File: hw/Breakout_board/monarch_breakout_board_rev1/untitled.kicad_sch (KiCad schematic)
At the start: 10 parts, among them J1 5037630491, J2 5037630291, J3 5037630291, J4 5037630291, J5 5037630291, J6 5037630291

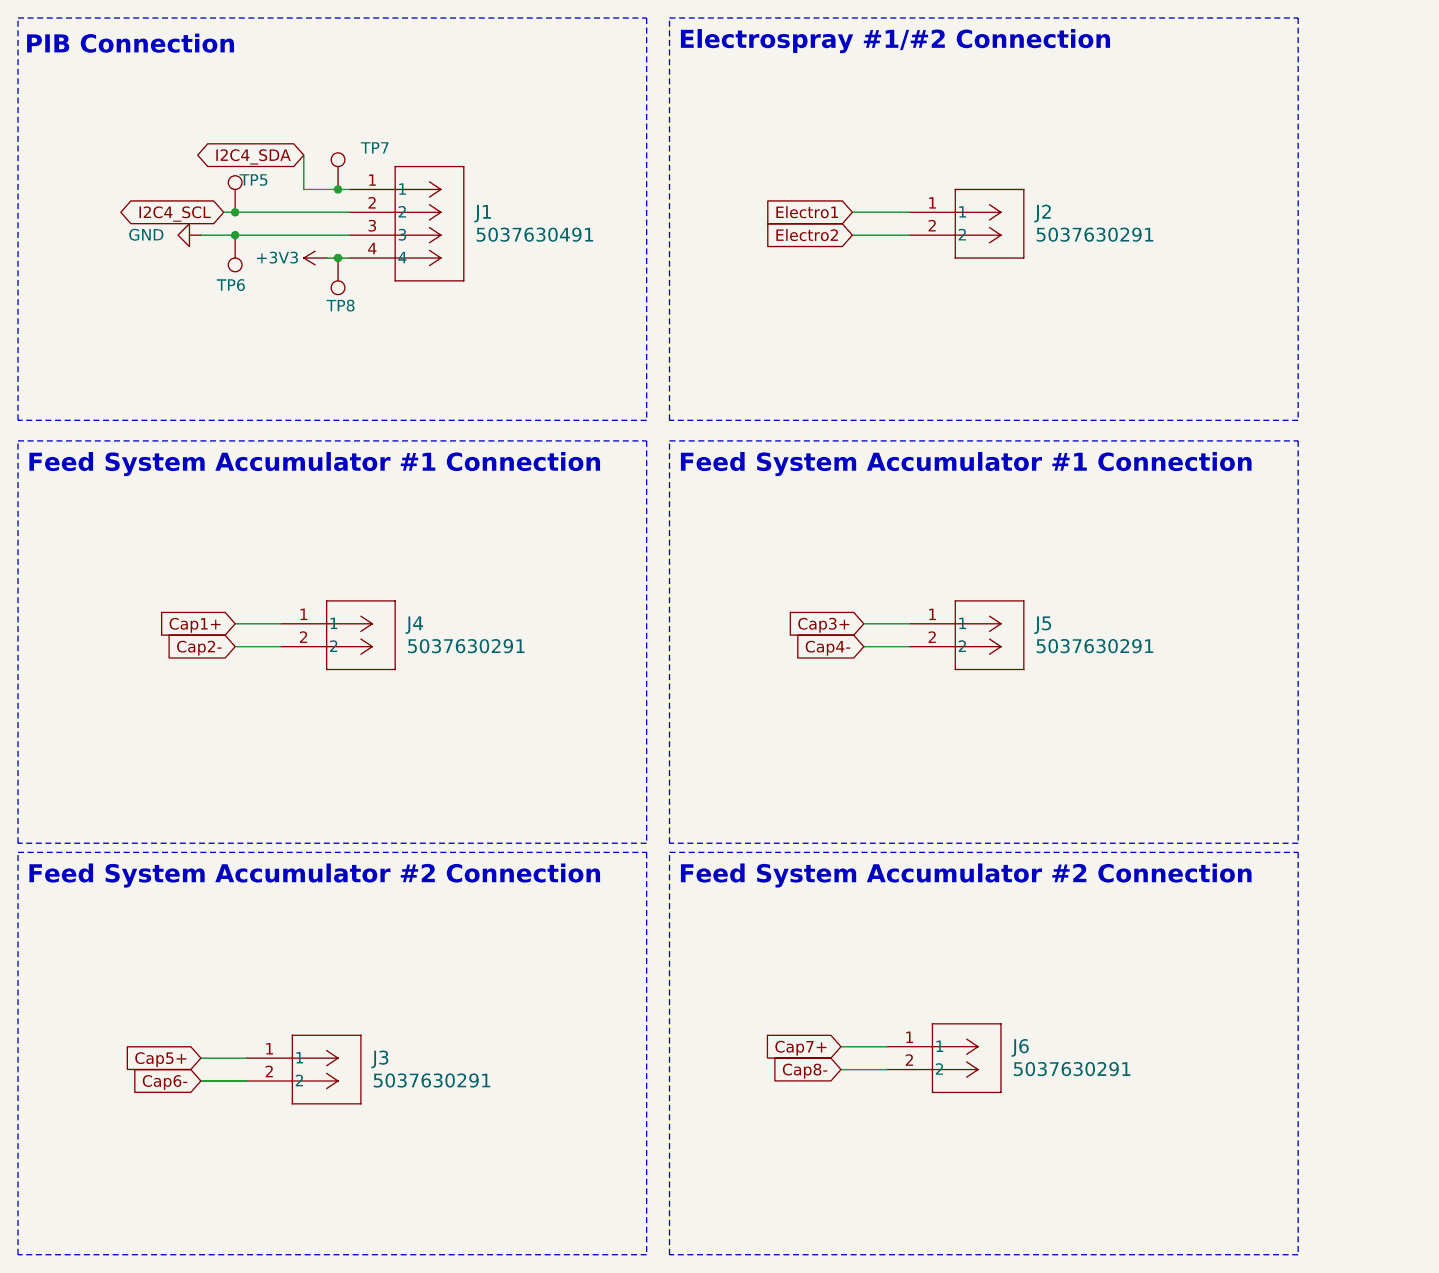
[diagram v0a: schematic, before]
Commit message: Revert "Crystal Clock Completion, All Pins Assigned, More Routing Work"
This reverts commit 432819c756e1f3cf9abb2627b488983cb7a3cfe3
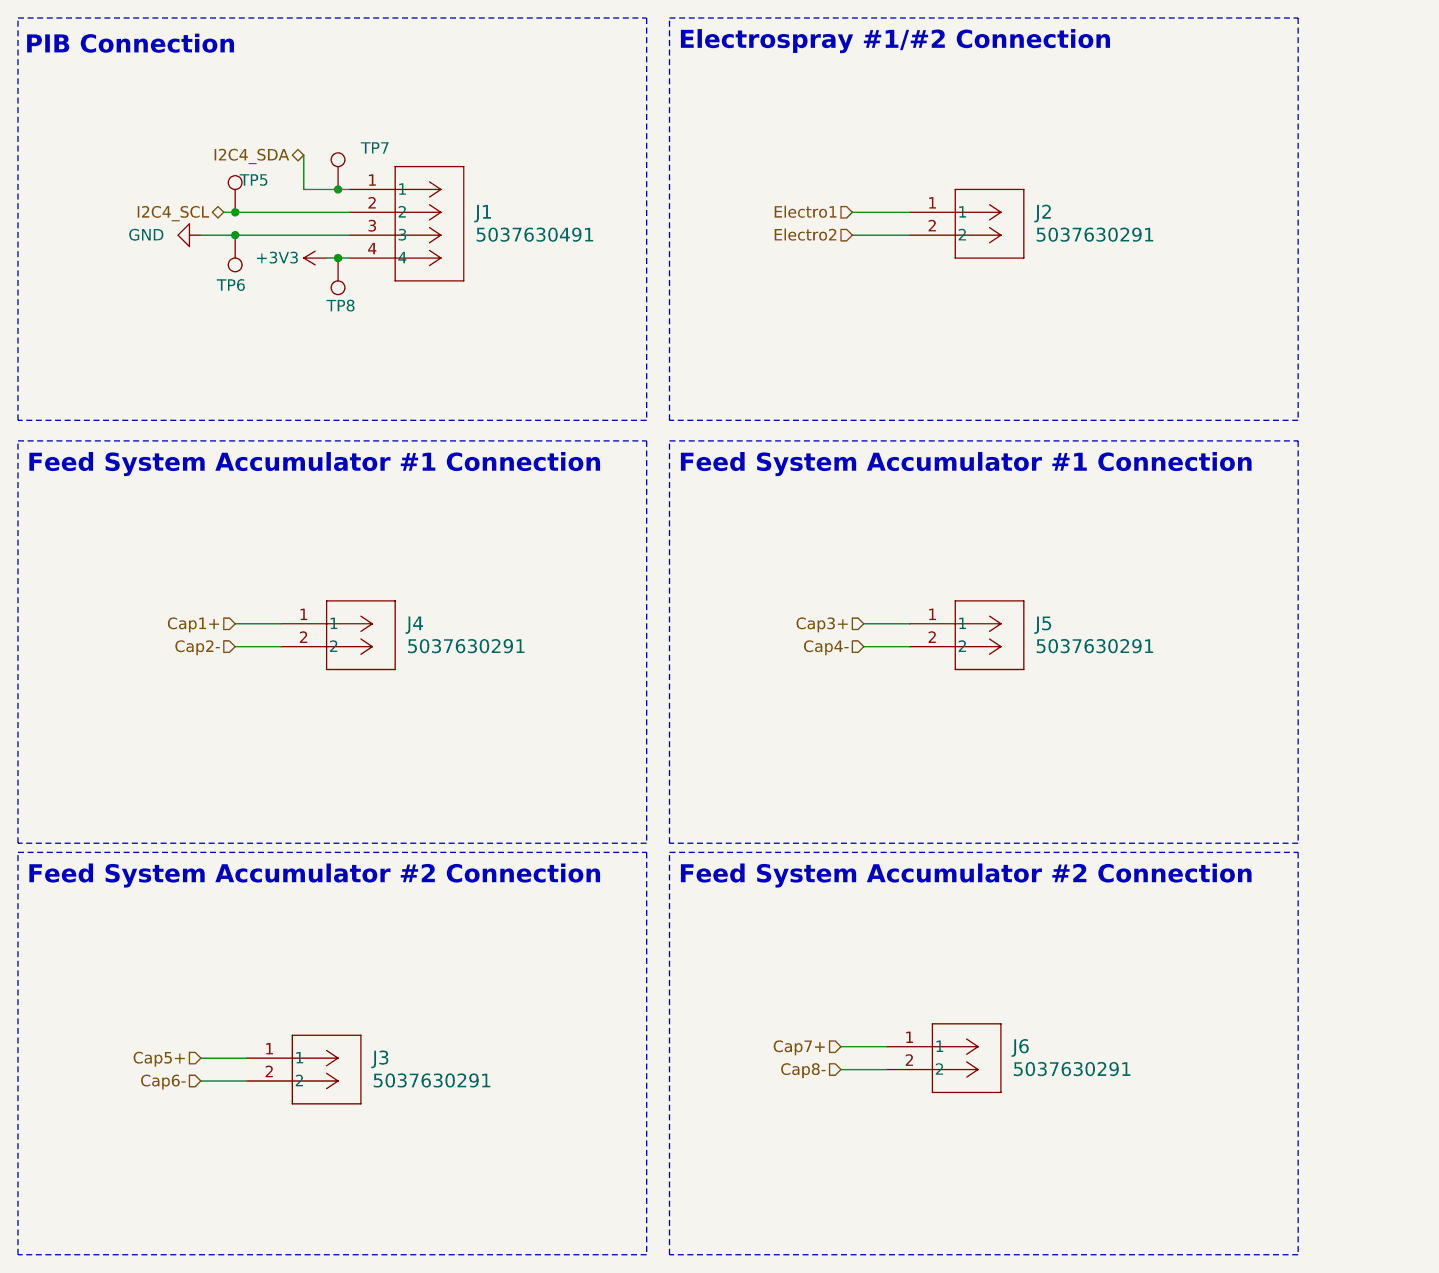
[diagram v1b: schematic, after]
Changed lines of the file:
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@@
 		)
 	)
-	(global_label "Cap1+"
+	(hierarchical_label "Cap5+"
 		(shape input)
-		(at 39.37 81.28 180)
-		(fields_autoplaced yes)
+		(at 35.56 129.54 180)
 		(effects
 			(font
@@
 			(justify right)
 		)
-		(property "Intersheetrefs" "${INTERSHEET_REFS}"
-			(at 30.0349 81.28 0)
-			(effects
-				(font
-					(size 1.27 1.27)
-				)
-				(justify right)
-				(hide yes)
-			)
-		)
 	)
-	(global_label "Electro2"
+	(hierarchical_label "Cap4-"
 		(shape input)
-		(at 107.95 38.1 180)
-		(fields_autoplaced yes)
+		(at 109.22 83.82 180)
 		(effects
 			(font
@@
 			(justify right)
 		)
-		(property "Intersheetrefs" "${INTERSHEET_REFS}"
-			(at 97.103 38.1 0)
-			(effects
-				(font
-					(size 1.27 1.27)
-				)
-				(justify right)
-				(hide yes)
-			)
-		)
 	)
-	(global_label "Cap4-"
-		(shape input)
-		(at 109.22 83.82 180)
-		(fields_autoplaced yes)
+	(hierarchical_label "I2C4_SCL"
+		(shape bidirectional)
+		(at 38.1 35.56 180)
 		(effects
 			(font
@@
 			(justify right)
 		)
-		(property "Intersheetrefs" "${INTERSHEET_REFS}"
-			(at 99.8849 83.82 0)
-			(effects
-				(font
-					(size 1.27 1.27)
-				)
-				(justify right)
-				(hide yes)
-			)
-		)
 	)
-	(global_label "Cap7+"
+	(hierarchical_label "Cap3+"
 		(shape input)
-		(at 106.68 128.27 180)
-		(fields_autoplaced yes)
+		(at 109.22 81.28 180)
 		(effects
 			(font
@@
 			(justify right)
 		)
-		(property "Intersheetrefs" "${INTERSHEET_REFS}"
-			(at 97.3449 128.27 0)
-			(effects
-				(font
-					(size 1.27 1.27)
-				)
-				(justify right)
-				(hide yes)
-			)
-		)
 	)
-	(global_label "Electro1"
+	(hierarchical_label "Electro2"
 		(shape input)
-		(at 107.95 35.56 180)
-		(fields_autoplaced yes)
+		(at 107.95 38.1 180)
 		(effects
 			(font
@@
 			(justify right)
 		)
-		(property "Intersheetrefs" "${INTERSHEET_REFS}"
-			(at 97.103 35.56 0)
-			(effects
-				(font
-					(size 1.27 1.27)
-				)
-				(justify right)
-				(hide yes)
-			)
-		)
 	)
-	(global_label "I2C4_SDA"
-		(shape bidirectional)
-		(at 46.99 29.21 180)
-		(fields_autoplaced yes)
+	(hierarchical_label "Cap2-"
+		(shape input)
+		(at 39.37 83.82 180)
 		(effects
 			(font
@@
 			(justify right)
 		)
-		(property "Intersheetrefs" "${INTERSHEET_REFS}"
-			(at 34.064 29.21 0)
-			(effects
-				(font
-					(size 1.27 1.27)
-				)
-				(justify right)
-				(hide yes)
-			)
-		)
 	)
-	(global_label "Cap3+"
+	(hierarchical_label "Cap6-"
 		(shape input)
-		(at 109.22 81.28 180)
-		(fields_autoplaced yes)
+		(at 35.56 132.08 180)
 		(effects
 			(font
@@
 			(justify right)
 		)
-		(property "Intersheetrefs" "${INTERSHEET_REFS}"
-			(at 99.8849 81.28 0)
-			(effects
-				(font
-					(size 1.27 1.27)
-				)
-				(justify right)
-				(hide yes)
-			)
-		)
 	)
-	(global_label "I2C4_SCL"
-		(shape bidirectional)
-		(at 38.1 35.56 180)
-		(fields_autoplaced yes)
+	(hierarchical_label "Cap8-"
+		(shape input)
+		(at 106.68 130.81 180)
 		(effects
 			(font
@@
 			(justify right)
 		)
-		(property "Intersheetrefs" "${INTERSHEET_REFS}"
-			(at 25.2345 35.56 0)
-			(effects
-				(font
-					(size 1.27 1.27)
-				)
-				(justify right)
-				(hide yes)
-			)
-		)
 	)
-	(global_label "Cap2-"
+	(hierarchical_label "Electro1"
 		(shape input)
-		(at 39.37 83.82 180)
-		(fields_autoplaced yes)
+		(at 107.95 35.56 180)
 		(effects
 			(font
@@
 			(justify right)
 		)
-		(property "Intersheetrefs" "${INTERSHEET_REFS}"
-			(at 30.0349 83.82 0)
-			(effects
-				(font
-					(size 1.27 1.27)
-				)
-				(justify right)
-				(hide yes)
-			)
-		)
 	)
-	(global_label "Cap5+"
+	(hierarchical_label "Cap7+"
 		(shape input)
-		(at 35.56 129.54 180)
-		(fields_autoplaced yes)
+		(at 106.68 128.27 180)
 		(effects
 			(font
@@
 			(justify right)
 		)
-		(property "Intersheetrefs" "${INTERSHEET_REFS}"
-			(at 26.2249 129.54 0)
-			(effects
-				(font
-					(size 1.27 1.27)
-				)
-				(justify right)
-				(hide yes)
-			)
-		)
 	)
-	(global_label "Cap8-"
+	(hierarchical_label "Cap1+"
 		(shape input)
-		(at 106.68 130.81 180)
-		(fields_autoplaced yes)
+		(at 39.37 81.28 180)
 		(effects
 			(font
@@
 			(justify right)
 		)
-		(property "Intersheetrefs" "${INTERSHEET_REFS}"
-			(at 97.3449 130.81 0)
-			(effects
-				(font
-					(size 1.27 1.27)
-				)
-				(justify right)
-				(hide yes)
-			)
-		)
 	)
-	(global_label "Cap6-"
-		(shape input)
-		(at 35.56 132.08 180)
-		(fields_autoplaced yes)
+	(hierarchical_label "I2C4_SDA"
+		(shape bidirectional)
+		(at 46.99 29.21 180)
 		(effects
 			(font
@@
 			(justify right)
 		)
-		(property "Intersheetrefs" "${INTERSHEET_REFS}"
-			(at 26.2249 132.08 0)
-			(effects
-				(font
-					(size 1.27 1.27)
-				)
-				(justify right)
-				(hide yes)
-			)
-		)
 	)

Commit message: Breakout Board History Fix
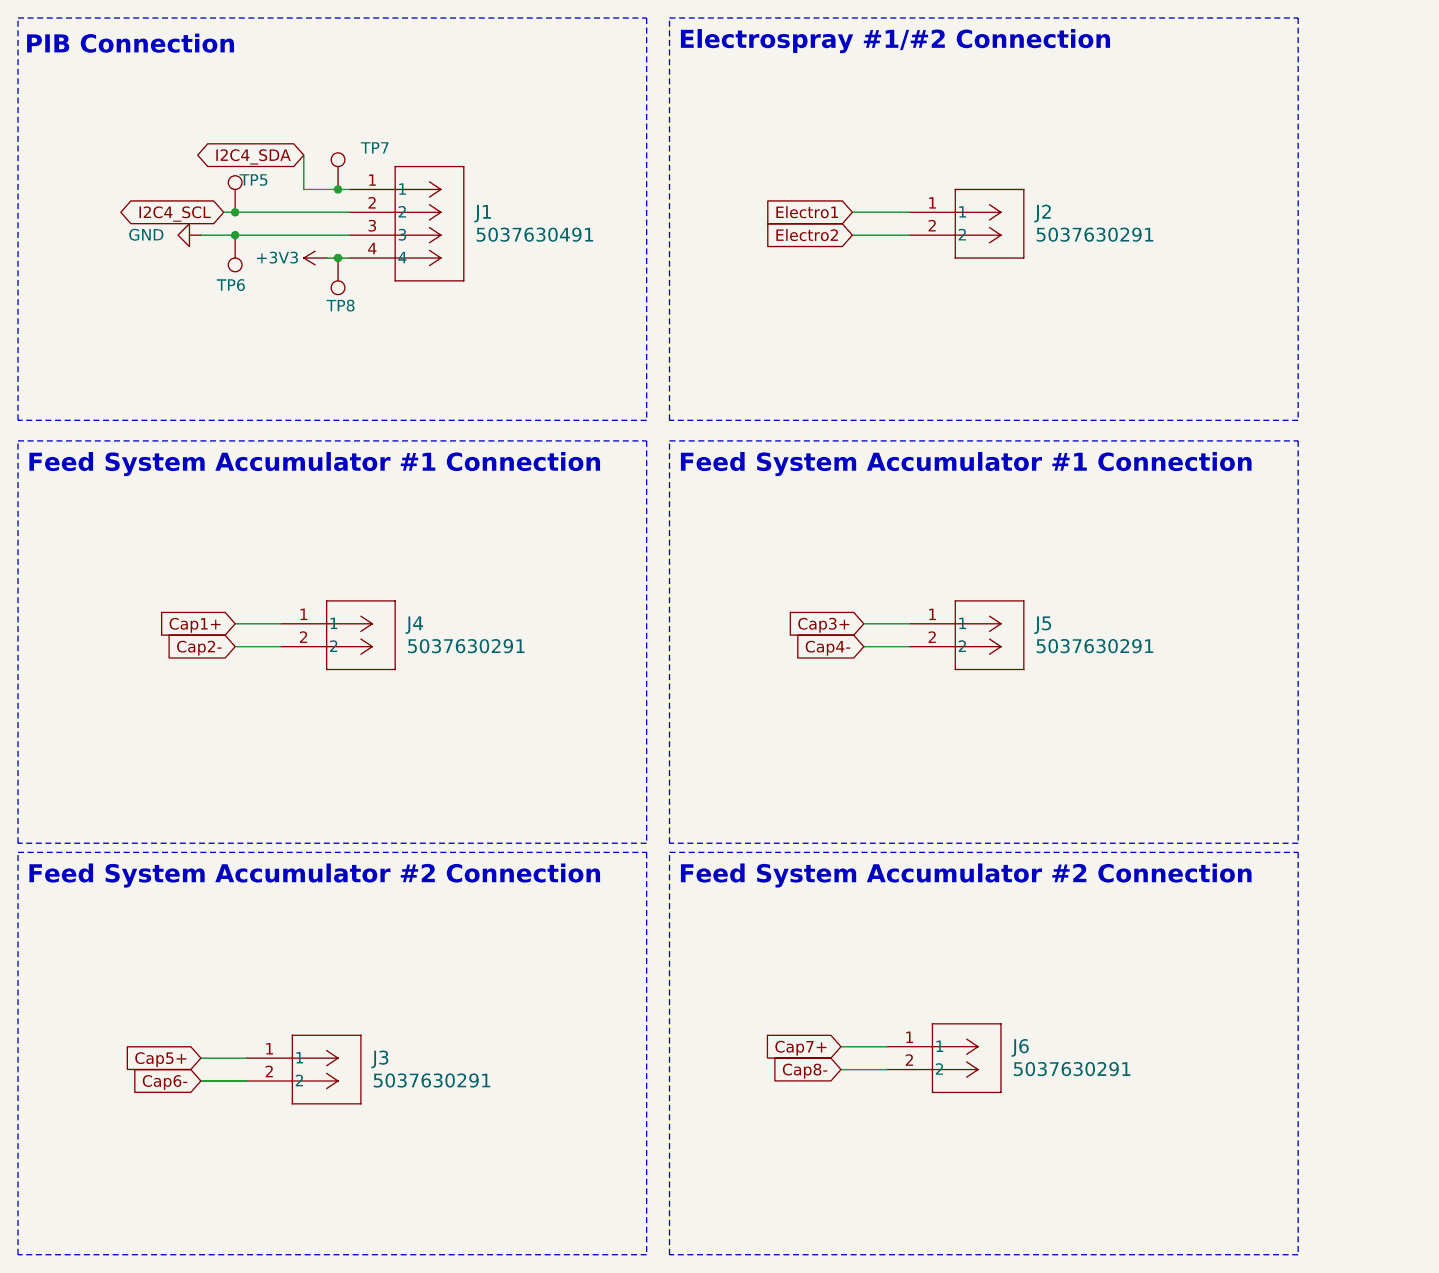
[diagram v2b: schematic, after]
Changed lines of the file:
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@@
 		)
 	)
-	(hierarchical_label "Cap5+"
-		(shape input)
-		(at 35.56 129.54 180)
-		(effects
-			(font
-				(size 1.27 1.27)
-			)
-			(justify right)
-		)
-	)
-	(hierarchical_label "Cap4-"
+	(global_label "Cap1+"
+		(shape input)
+		(at 39.37 81.28 180)
+		(fields_autoplaced yes)
+		(effects
+			(font
+				(size 1.27 1.27)
+			)
+			(justify right)
+		)
+		(property "Intersheetrefs" "${INTERSHEET_REFS}"
+			(at 30.0349 81.28 0)
+			(effects
+				(font
+					(size 1.27 1.27)
+				)
+				(justify right)
+				(hide yes)
+			)
+		)
+	)
+	(global_label "Electro2"
+		(shape input)
+		(at 107.95 38.1 180)
+		(fields_autoplaced yes)
+		(effects
+			(font
+				(size 1.27 1.27)
+			)
+			(justify right)
+		)
+		(property "Intersheetrefs" "${INTERSHEET_REFS}"
+			(at 97.103 38.1 0)
+			(effects
+				(font
+					(size 1.27 1.27)
+				)
+				(justify right)
+				(hide yes)
+			)
+		)
+	)
+	(global_label "Cap4-"
 		(shape input)
 		(at 109.22 83.82 180)
-		(effects
-			(font
-				(size 1.27 1.27)
-			)
-			(justify right)
-		)
-	)
-	(hierarchical_label "I2C4_SCL"
+		(fields_autoplaced yes)
+		(effects
+			(font
+				(size 1.27 1.27)
+			)
+			(justify right)
+		)
+		(property "Intersheetrefs" "${INTERSHEET_REFS}"
+			(at 99.8849 83.82 0)
+			(effects
+				(font
+					(size 1.27 1.27)
+				)
+				(justify right)
+				(hide yes)
+			)
+		)
+	)
+	(global_label "Cap7+"
+		(shape input)
+		(at 106.68 128.27 180)
+		(fields_autoplaced yes)
+		(effects
+			(font
+				(size 1.27 1.27)
+			)
+			(justify right)
+		)
+		(property "Intersheetrefs" "${INTERSHEET_REFS}"
+			(at 97.3449 128.27 0)
+			(effects
+				(font
+					(size 1.27 1.27)
+				)
+				(justify right)
+				(hide yes)
+			)
+		)
+	)
+	(global_label "Electro1"
+		(shape input)
+		(at 107.95 35.56 180)
+		(fields_autoplaced yes)
+		(effects
+			(font
+				(size 1.27 1.27)
+			)
+			(justify right)
+		)
+		(property "Intersheetrefs" "${INTERSHEET_REFS}"
+			(at 97.103 35.56 0)
+			(effects
+				(font
+					(size 1.27 1.27)
+				)
+				(justify right)
+				(hide yes)
+			)
+		)
+	)
+	(global_label "I2C4_SDA"
+		(shape bidirectional)
+		(at 46.99 29.21 180)
+		(fields_autoplaced yes)
+		(effects
+			(font
+				(size 1.27 1.27)
+			)
+			(justify right)
+		)
+		(property "Intersheetrefs" "${INTERSHEET_REFS}"
+			(at 34.064 29.21 0)
+			(effects
+				(font
+					(size 1.27 1.27)
+				)
+				(justify right)
+				(hide yes)
+			)
+		)
+	)
+	(global_label "Cap3+"
+		(shape input)
+		(at 109.22 81.28 180)
+		(fields_autoplaced yes)
+		(effects
+			(font
+				(size 1.27 1.27)
+			)
+			(justify right)
+		)
+		(property "Intersheetrefs" "${INTERSHEET_REFS}"
+			(at 99.8849 81.28 0)
+			(effects
+				(font
+					(size 1.27 1.27)
+				)
+				(justify right)
+				(hide yes)
+			)
+		)
+	)
+	(global_label "I2C4_SCL"
 		(shape bidirectional)
 		(at 38.1 35.56 180)
-		(effects
-			(font
-				(size 1.27 1.27)
-			)
-			(justify right)
-		)
-	)
-	(hierarchical_label "Cap3+"
-		(shape input)
-		(at 109.22 81.28 180)
-		(effects
-			(font
-				(size 1.27 1.27)
-			)
-			(justify right)
-		)
-	)
-	(hierarchical_label "Electro2"
-		(shape input)
-		(at 107.95 38.1 180)
-		(effects
-			(font
-				(size 1.27 1.27)
-			)
-			(justify right)
-		)
-	)
-	(hierarchical_label "Cap2-"
+		(fields_autoplaced yes)
+		(effects
+			(font
+				(size 1.27 1.27)
+			)
+			(justify right)
+		)
+		(property "Intersheetrefs" "${INTERSHEET_REFS}"
+			(at 25.2345 35.56 0)
+			(effects
+				(font
+					(size 1.27 1.27)
+				)
+				(justify right)
+				(hide yes)
+			)
+		)
+	)
+	(global_label "Cap2-"
 		(shape input)
 		(at 39.37 83.82 180)
-		(effects
-			(font
-				(size 1.27 1.27)
-			)
-			(justify right)
-		)
-	)
-	(hierarchical_label "Cap6-"
+		(fields_autoplaced yes)
+		(effects
+			(font
+				(size 1.27 1.27)
+			)
+			(justify right)
+		)
+		(property "Intersheetrefs" "${INTERSHEET_REFS}"
+			(at 30.0349 83.82 0)
+			(effects
+				(font
+					(size 1.27 1.27)
+				)
+				(justify right)
+				(hide yes)
+			)
+		)
+	)
+	(global_label "Cap5+"
+		(shape input)
+		(at 35.56 129.54 180)
+		(fields_autoplaced yes)
+		(effects
+			(font
+				(size 1.27 1.27)
+			)
+			(justify right)
+		)
+		(property "Intersheetrefs" "${INTERSHEET_REFS}"
+			(at 26.2249 129.54 0)
+			(effects
+				(font
+					(size 1.27 1.27)
+				)
+				(justify right)
+				(hide yes)
+			)
+		)
+	)
+	(global_label "Cap8-"
+		(shape input)
+		(at 106.68 130.81 180)
+		(fields_autoplaced yes)
+		(effects
+			(font
+				(size 1.27 1.27)
+			)
+			(justify right)
+		)
+		(property "Intersheetrefs" "${INTERSHEET_REFS}"
+			(at 97.3449 130.81 0)
+			(effects
+				(font
+					(size 1.27 1.27)
+				)
+				(justify right)
+				(hide yes)
+			)
+		)
+	)
+	(global_label "Cap6-"
 		(shape input)
 		(at 35.56 132.08 180)
-		(effects
-			(font
-				(size 1.27 1.27)
-			)
-			(justify right)
-		)
-	)
-	(hierarchical_label "Cap8-"
-		(shape input)
-		(at 106.68 130.81 180)
-		(effects
-			(font
-				(size 1.27 1.27)
-			)
-			(justify right)
-		)
-	)
-	(hierarchical_label "Electro1"
-		(shape input)
-		(at 107.95 35.56 180)
-		(effects
-			(font
-				(size 1.27 1.27)
-			)
-			(justify right)
-		)
-	)
-	(hierarchical_label "Cap7+"
-		(shape input)
-		(at 106.68 128.27 180)
-		(effects
-			(font
-				(size 1.27 1.27)
-			)
-			(justify right)
-		)
-	)
-	(hierarchical_label "Cap1+"
-		(shape input)
-		(at 39.37 81.28 180)
-		(effects
-			(font
-				(size 1.27 1.27)
-			)
-			(justify right)
-		)
-	)
-	(hierarchical_label "I2C4_SDA"
-		(shape bidirectional)
-		(at 46.99 29.21 180)
-		(effects
-			(font
-				(size 1.27 1.27)
-			)
-			(justify right)
-		)
-	)
+		(fields_autoplaced yes)
+		(effects
+			(font
+				(size 1.27 1.27)
+			)
+			(justify right)
+		)
+		(property "Intersheetrefs" "${INTERSHEET_REFS}"
+			(at 26.2249 132.08 0)
+			(effects
+				(font
+					(size 1.27 1.27)
+				)
+				(justify right)
+				(hide yes)
+			)
+		)
+	)
